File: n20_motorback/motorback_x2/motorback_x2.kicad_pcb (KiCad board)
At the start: 2 copper layers, 19.9 x 11 mm, 13 parts, among them J1 Servo wire input, J2 Conn_01x01_Male, J3 Conn_01x01_Male, J4 prog_pins, U1 DRV8837DSGR, U2 ATtiny4-TS, U3 AIC1734-33GUTR

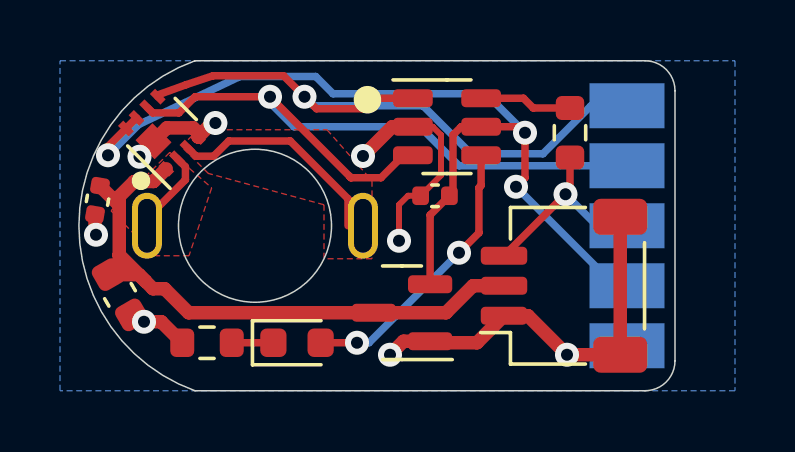
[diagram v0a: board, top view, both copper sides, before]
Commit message: mechanical improvements
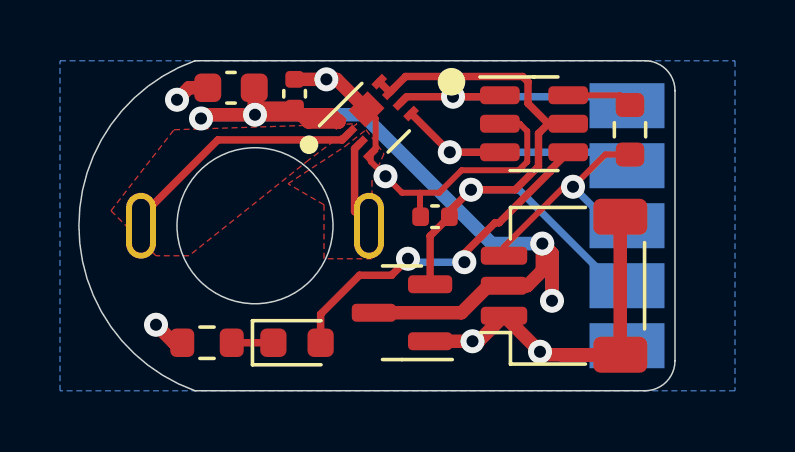
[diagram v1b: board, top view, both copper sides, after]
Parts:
- moved C1 7.83 mm to (159.2, 115.4), turned to 180 degrees
- moved C2 7.47 mm to (161.3, 115.6), turned to 90 degrees
- moved U1 7.12 mm to (164.0, 116.4), turned to 45 degrees
- moved U2 2.90 mm to (169.3, 116.6)
- moved R2 2.00 mm to (172.5, 116.8)
- moved C3 0.70 mm to (166.0, 119.7)
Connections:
- J4 pad 4: /MOTORF -> /MOTORR
- J4 pad 5: /MOTORR -> /MOTORF
- U2 pad 1: /MOTORR -> /MOTORF
- U2 pad 3: /MOTORF -> /MOTORR
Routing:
- net /MOTORF: track 23.6 -> 9.34 mm
- net VBAT: track 20.9 -> 33.1 mm, vias 0 -> 4
- net /MOTORR: track 21.5 -> 9.59 mm
- net /VLOGIC: track 32.0 -> 22.1 mm, vias 3 -> 1
- net /MOTOROUT1: track 2.90 -> 8.41 mm
- net /MOTOROUT2: track 7.38 -> 3.03 mm
- net GND: track 26.5 -> 29.8 mm, vias 8 -> 6
- net BLINKY: track 9.41 -> 11.7 mm
- net PWMIN: track 6.67 -> 8.11 mm
- net /PWMR: track 3.10 -> 2.20 mm
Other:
- outline, holes or cut-outs redrawn
